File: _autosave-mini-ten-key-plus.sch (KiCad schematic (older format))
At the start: 65 parts, among them SW0 SW_Push, U0 ProMicro

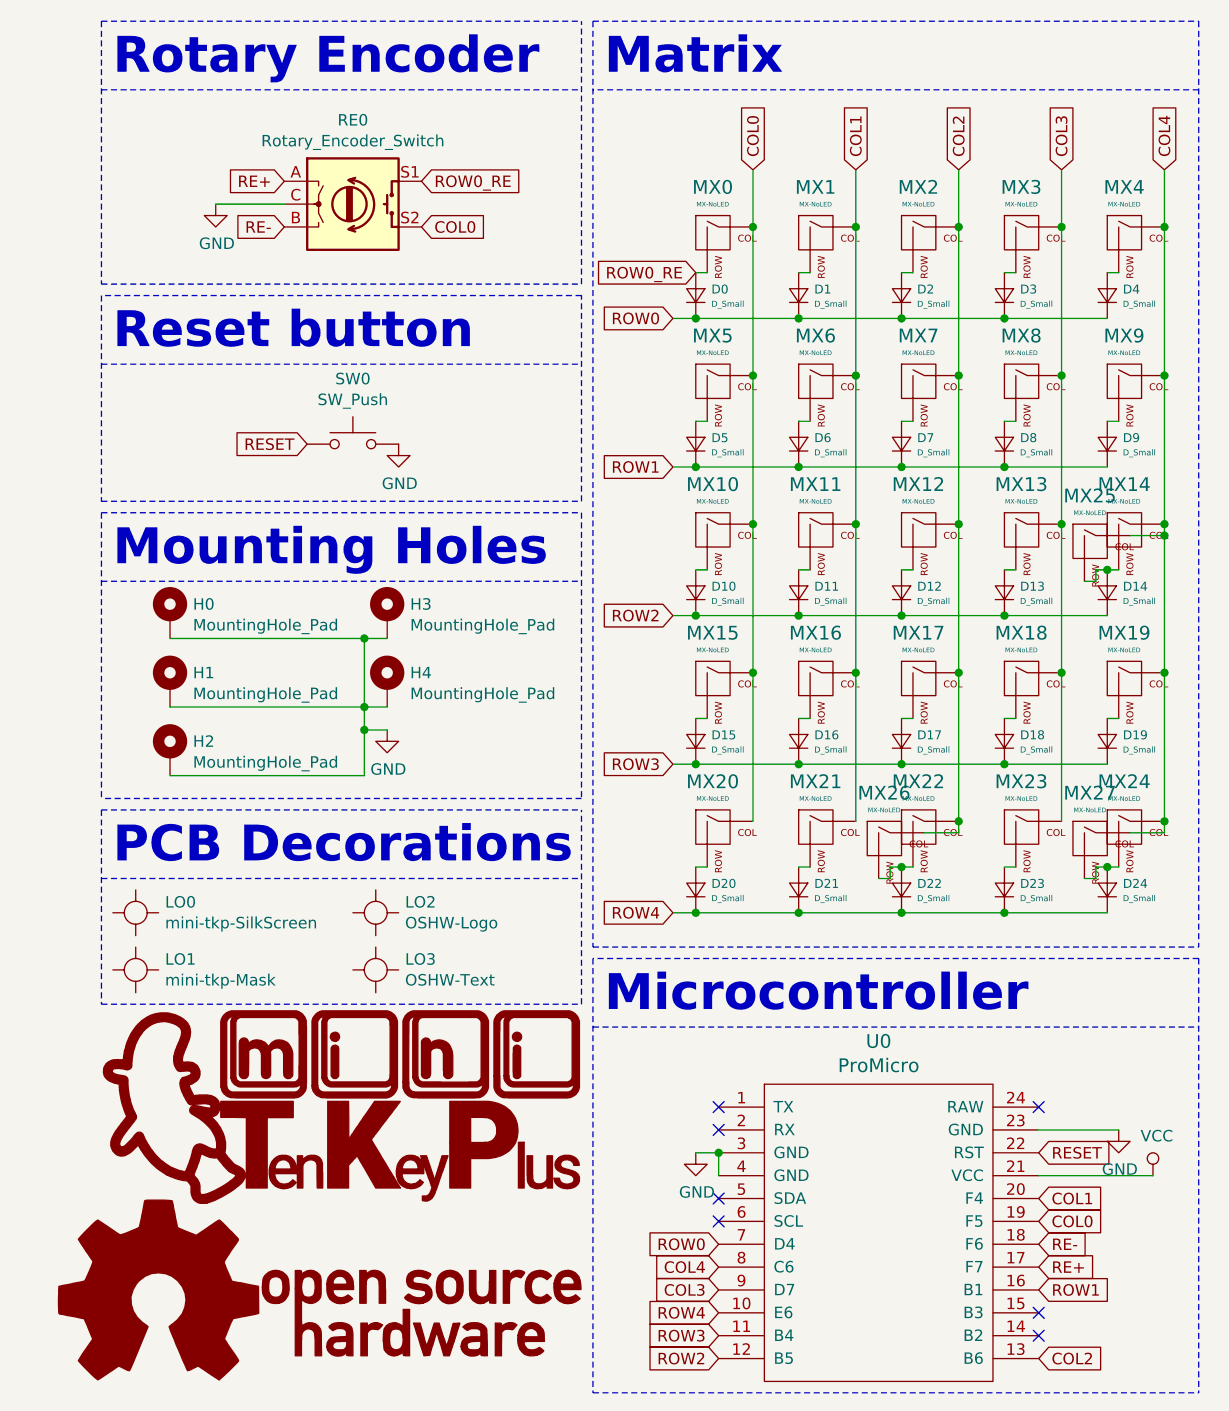
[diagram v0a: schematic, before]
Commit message: Added LICENSE
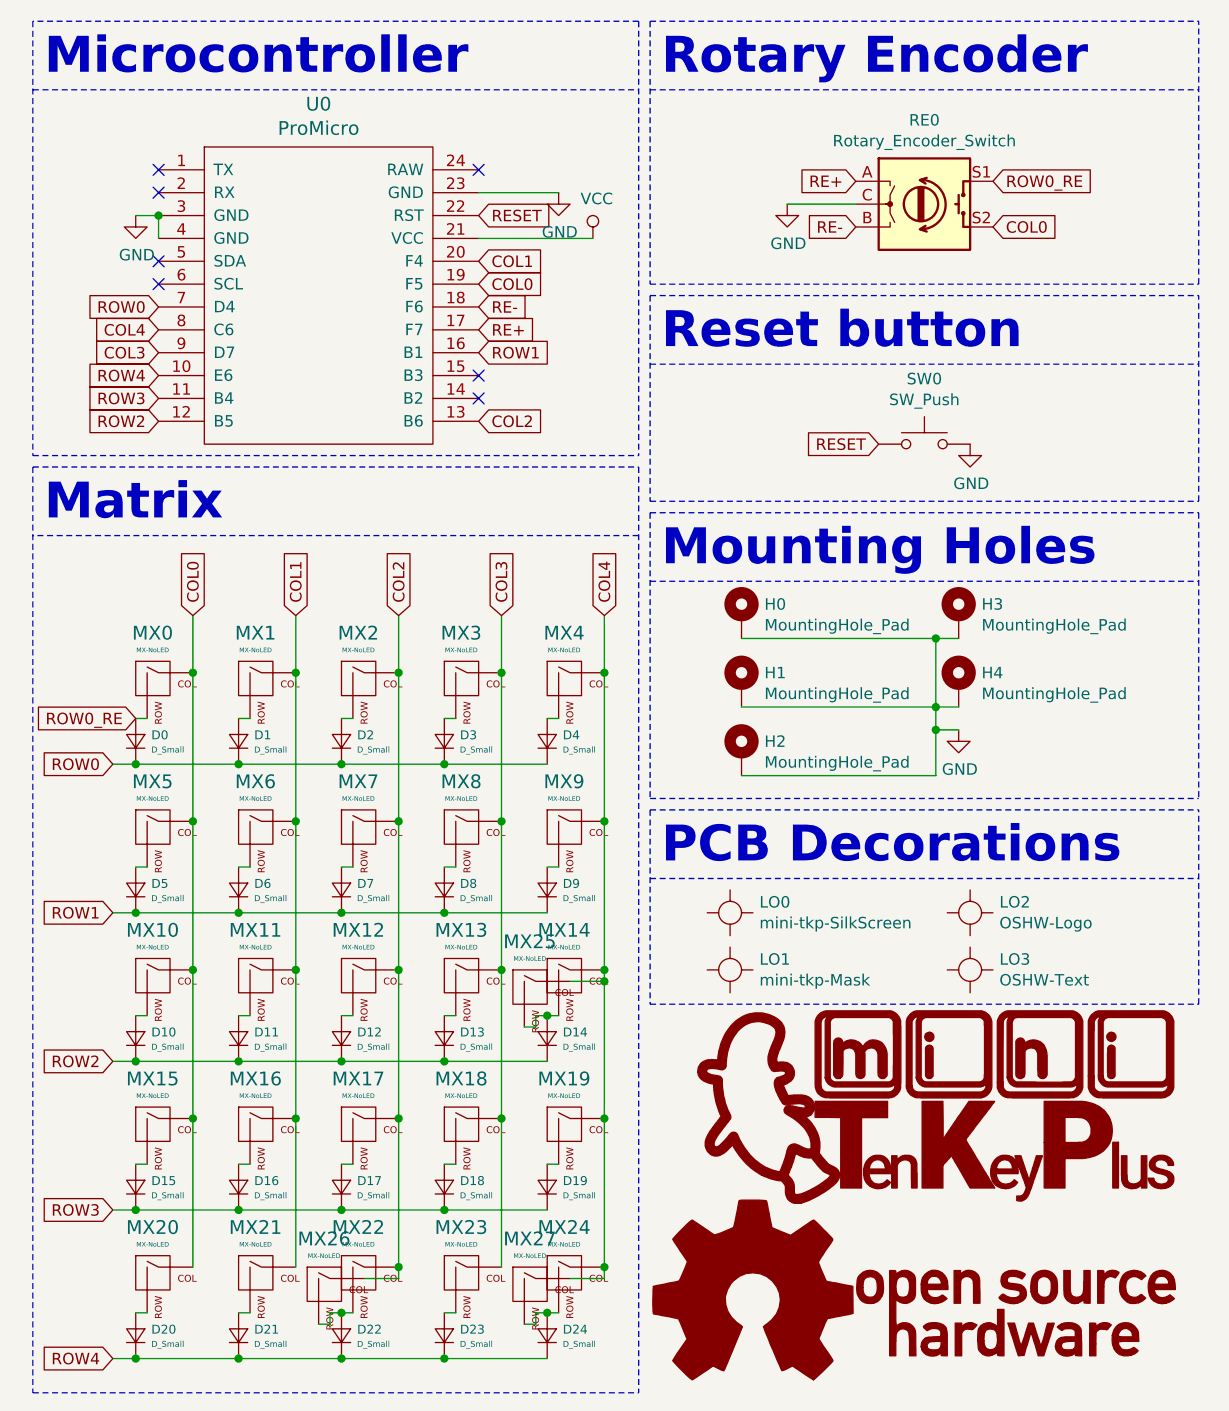
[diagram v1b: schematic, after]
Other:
- moved on the sheet: D0, D1, D10, D11, D12, D13, D14, D15, D16, D17, D18, D19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
